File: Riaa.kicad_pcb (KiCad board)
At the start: 2 copper layers, 44 parts, among them J1 power, J2 in, J3 out, U1 TL071, U2 TL072, U3 TL071, U4 TL071

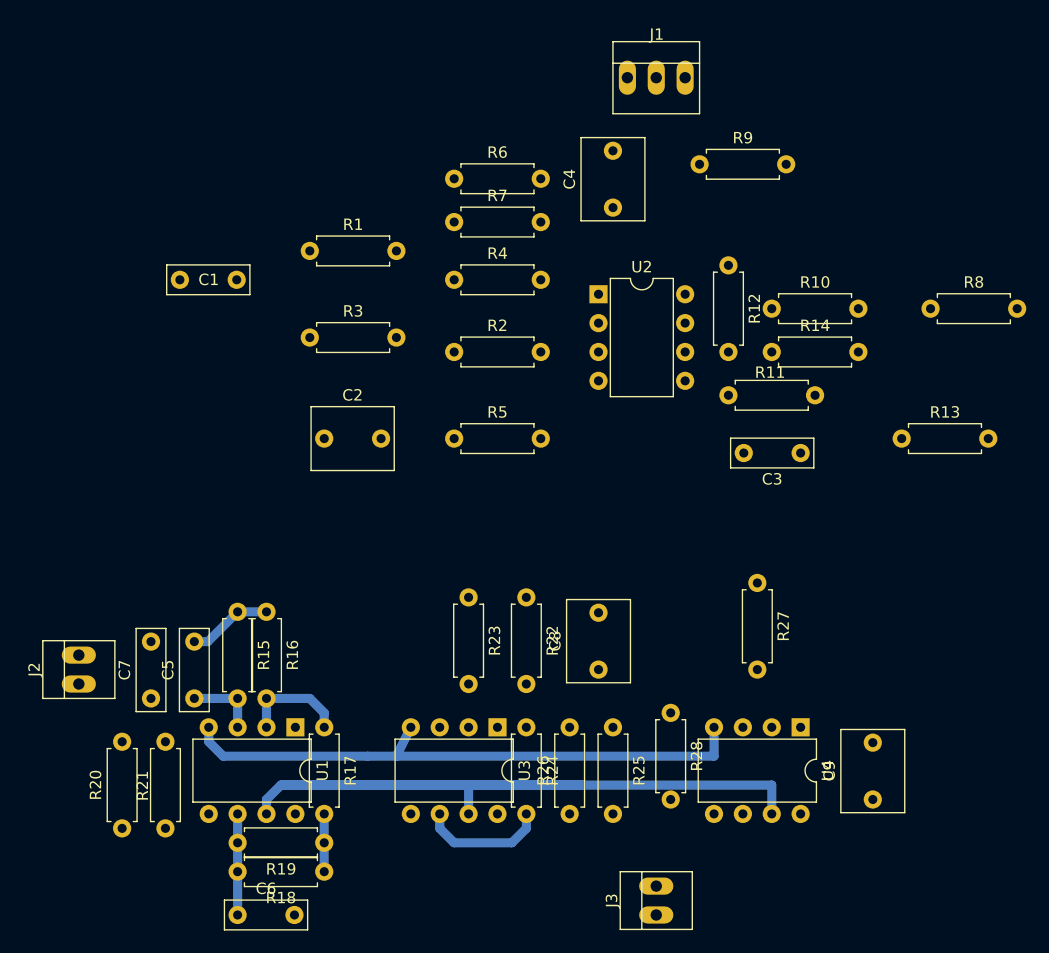
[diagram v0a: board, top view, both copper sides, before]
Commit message: decoupling
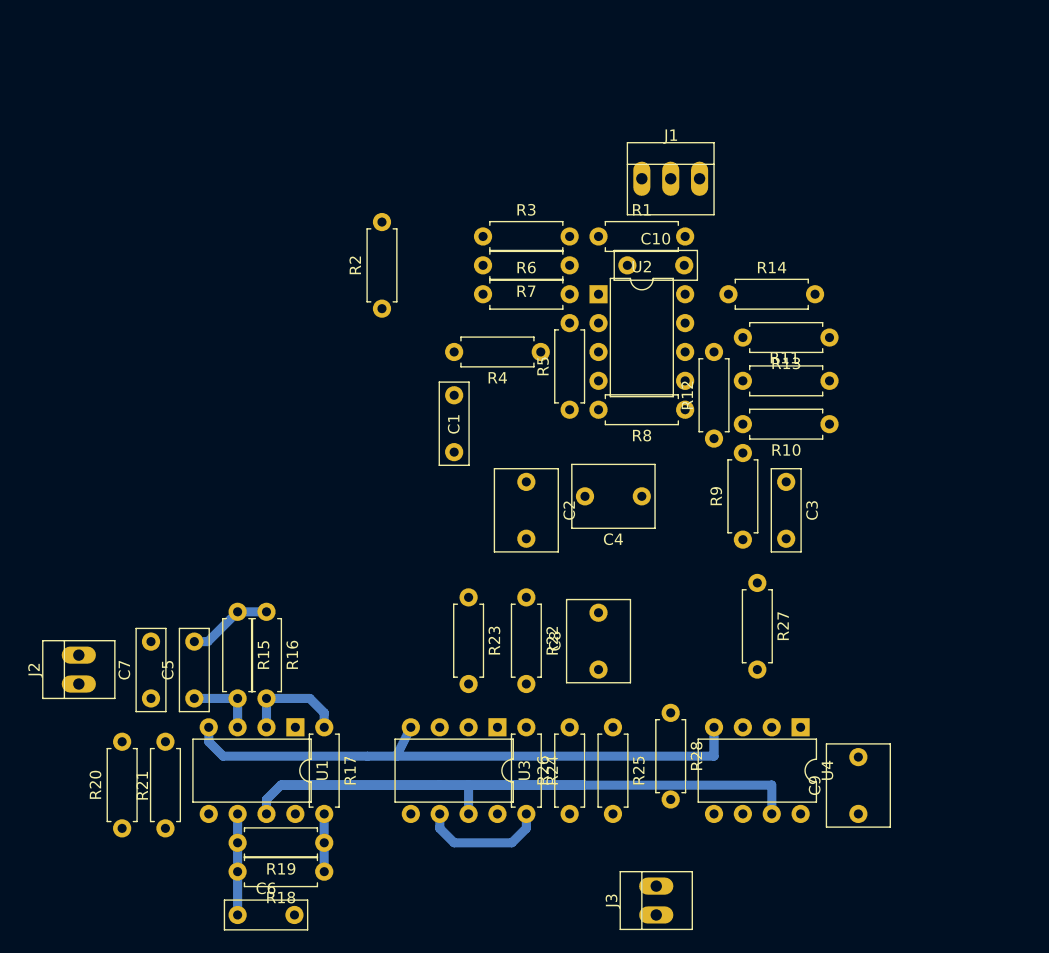
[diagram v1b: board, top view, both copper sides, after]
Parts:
- added C10: 100n, Capacitors_THT:C_Rect_L7.2mm_W2.5mm_P5.00mm_FKS2_FKP2_MKS2_MKP2, F.Cu at (67.3, 53.3)
- moved R9 33.2 mm to (77.5, 77.5), turned to 90 degrees
- moved C1 26.2 mm to (52.1, 64.8), turned to 270 degrees
- moved C4 25.5 mm to (68.6, 73.7), turned to 180 degrees
- moved R1 25.4 mm to (64.8, 50.8)
- moved R8 23.3 mm to (72.4, 66.0), turned to 180 degrees
- moved C2 18.2 mm to (58.4, 72.4), turned to 270 degrees
- moved R3 17.6 mm to (54.6, 50.8)
- moved R12 15.3 mm to (74.9, 68.6), turned to 90 degrees
- moved R10 11.4 mm to (85.1, 67.3), turned to 180 degrees
- moved R13 10.9 mm to (85.1, 59.7), turned to 180 degrees
- moved R7 10.9 mm to (62.2, 53.3), turned to 180 degrees
- moved R6 10.5 mm to (54.6, 55.9)
- moved R5 10.5 mm to (62.2, 66.0), turned to 90 degrees
- moved R4 9.92 mm to (59.7, 61.0), turned to 180 degrees
- moved J1 8.98 mm to (68.6, 45.7)
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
